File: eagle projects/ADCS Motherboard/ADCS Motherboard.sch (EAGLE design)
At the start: 145 parts, among them J1 HDR_10_EZFET_DEBUGGER, J11 CNC_3221-10-0300-00, J2A 832-10-012-10-005000, J2B 832-10-012-10-005000, J5 CNC_3221-10-0300-00, J7 TE-1734829-3, Q1 BSR802NL6327HTSA1, U1 MSP430F5529IPN, U10 TSV991AILT, U2 TSV991AILT, U3 ADS7841E_2K5, U4 TSV991AILT, U5 DMC4050SSDQ-13, U6 BNO055, U7 HMC1053, U9 BMX160, Y1 32.768kHz, Y2 CSTCR4M00G15L99, Y3 32.768kHz

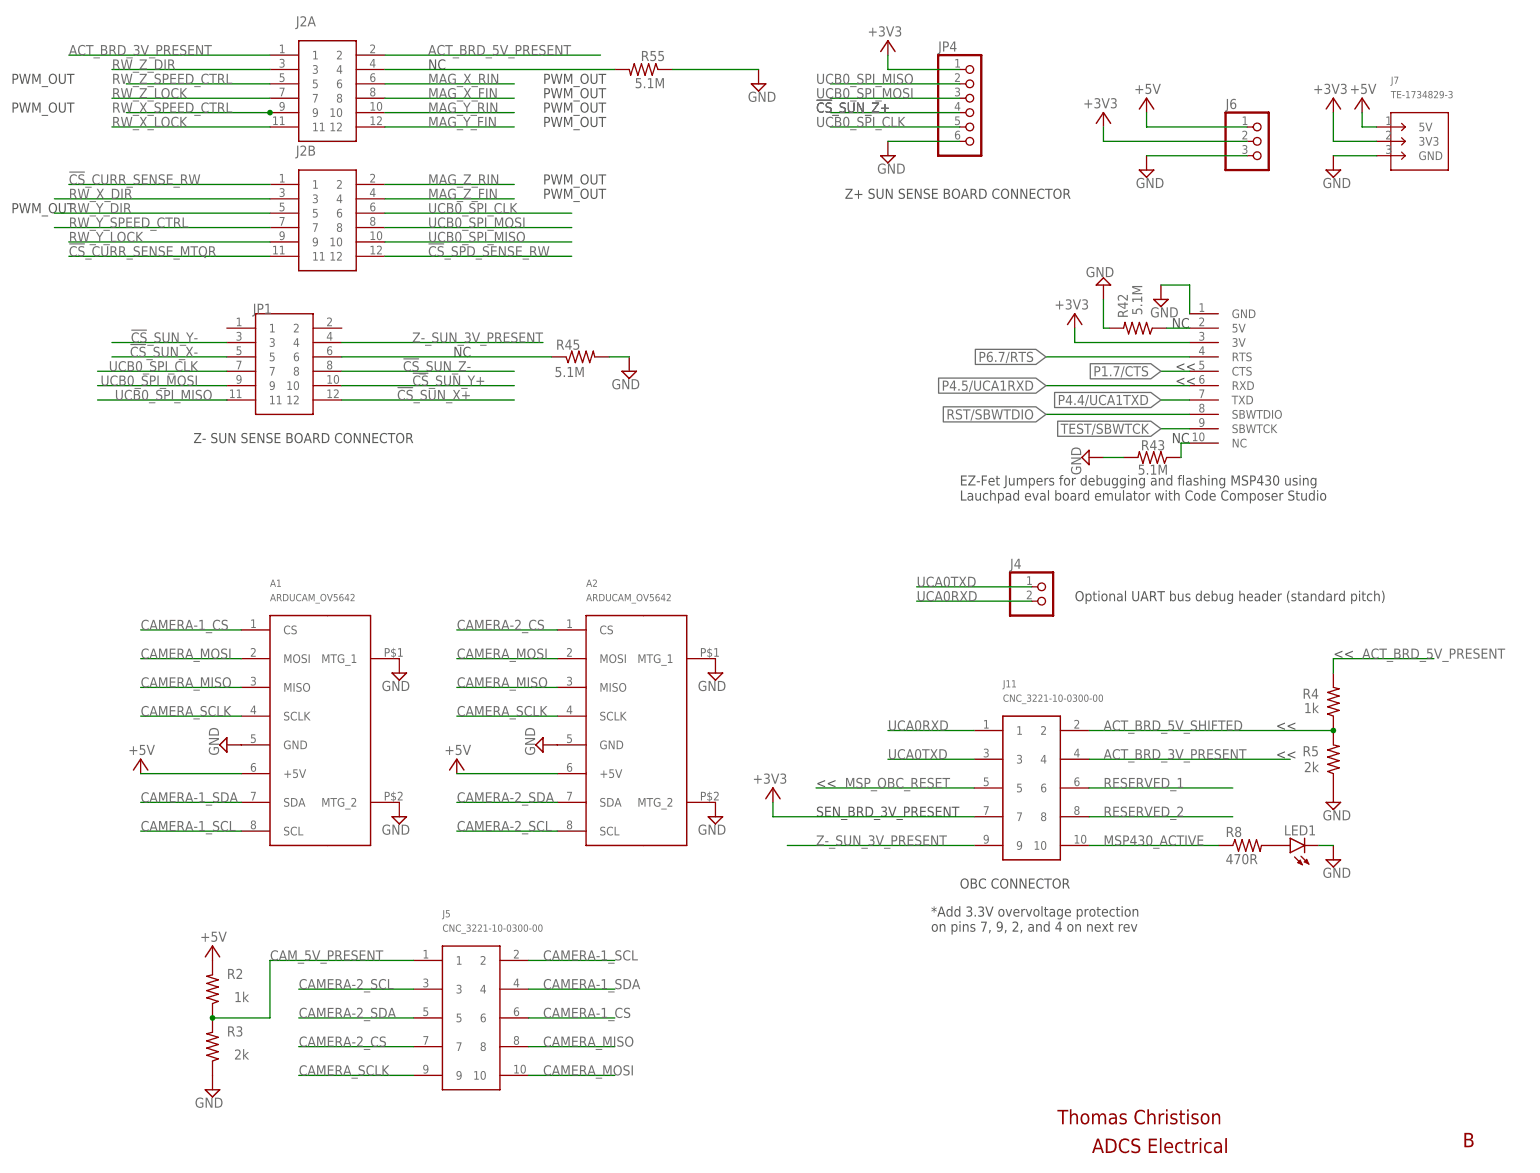
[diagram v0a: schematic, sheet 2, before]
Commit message: Finished all new connectors
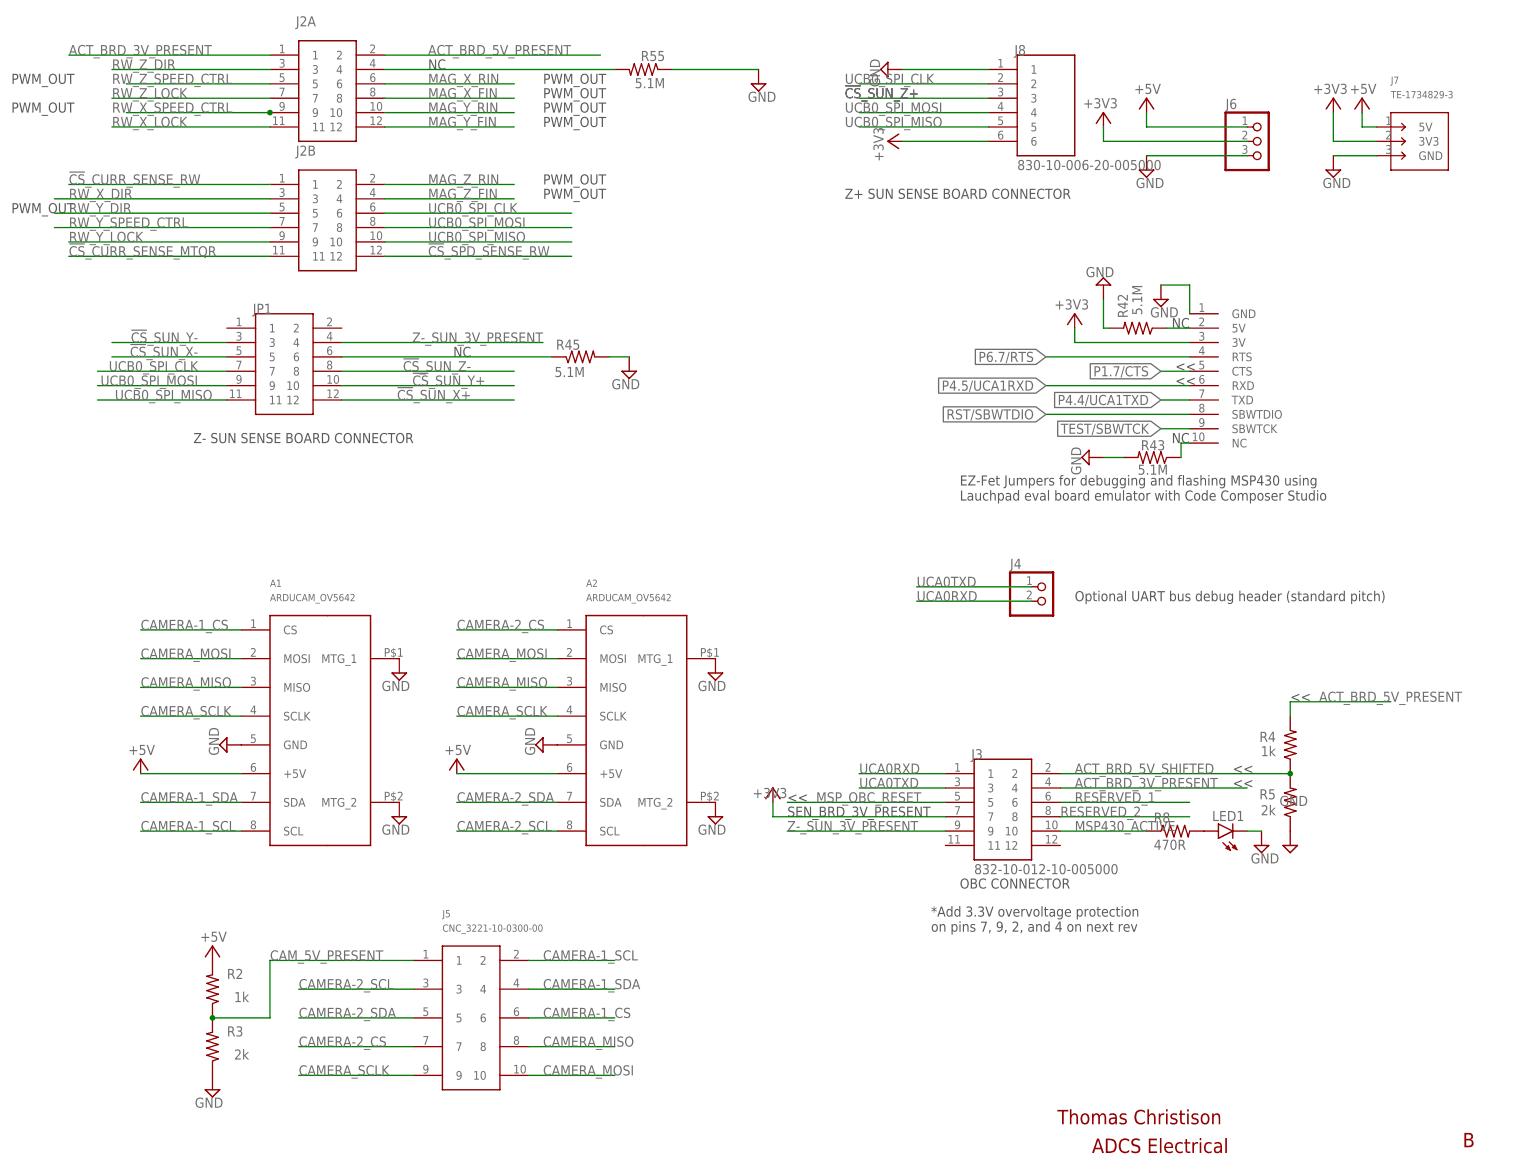
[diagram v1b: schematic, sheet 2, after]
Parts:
- removed J11: CNC_3221-10-0300-00, my_library:CNC_3221-10-0300-00
- removed JP4: (no value), my_library:PINHD-1X6
- added J3: 832-10-012-10-005000, 832-10-012-10-005000:832-10-012-10-005000
- added J8: 830-10-006-20-005000, 830-10-006-20-005000:830-10-006-20-005000
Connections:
- net !CS!_SUN_Z+: now also J8.3; no longer JP4.4
- net +3V3: now also J3.7, J8.6; no longer J11.7, JP4.1
- net ACT_BRD_3V_PRESENT: now also J3.4; no longer J11.4
- net ACT_BRD_5V_SHIFTED: now also J3.2; no longer J11.2
- net GND: now also J8.1; no longer JP4.6
- net MSP430_ACTIVE: now also J3.10; no longer J11.10
- net MSP_OBC_RESET: now also J3.5; no longer J11.5
- net RESERVED_1: now also J3.6; no longer J11.6
- net RESERVED_2: now also J3.8; no longer J11.8
- net UCA0RXD: now also J3.1; no longer J11.1
- net UCA0TXD: now also J3.3; no longer J11.3
- net UCB0_SPI_CLK: now also J8.2; no longer JP4.5
- net UCB0_SPI_MISO: now also J8.5; no longer JP4.2
- net UCB0_SPI_MOSI: now also J8.4; no longer JP4.3
- net Z-_SUN_3V_PRESENT: now also J3.9; no longer J11.9
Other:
- moved on the sheet: LED1, R4, R5, R8
